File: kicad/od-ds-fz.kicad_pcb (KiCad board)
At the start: 2 copper layers, 42 parts, among them J1 AudioJack2, J2 AudioJack2, U1 TLC274

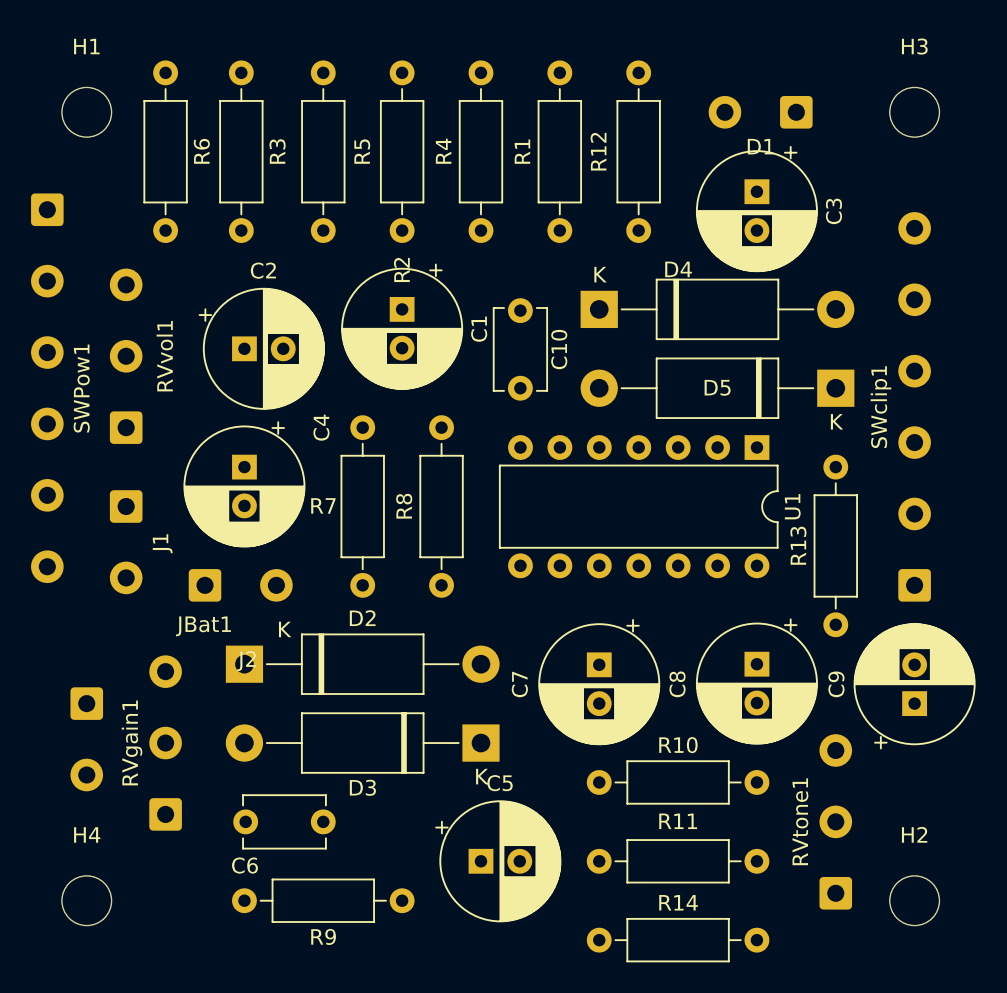
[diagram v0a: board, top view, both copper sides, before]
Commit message: Precise placement
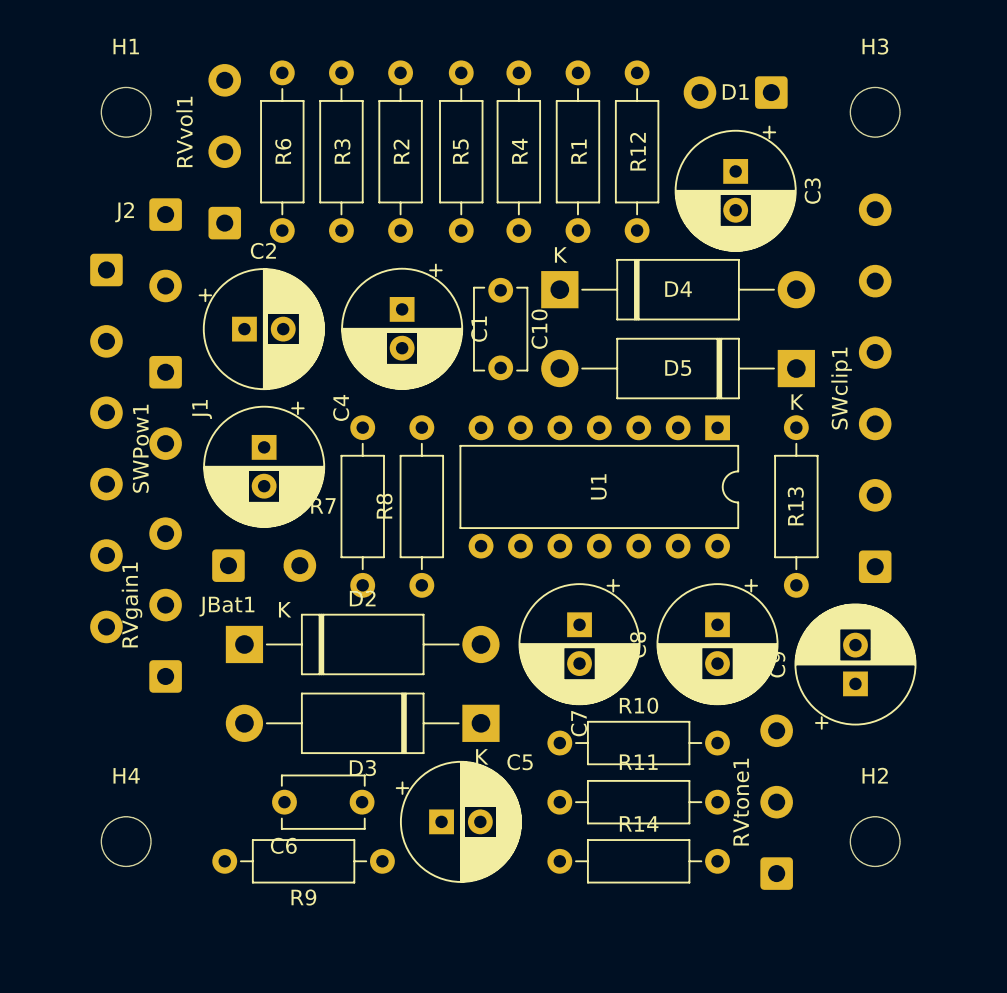
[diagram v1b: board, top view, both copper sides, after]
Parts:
- moved J2 31.9 mm to (127.0, 67.5)
- moved RVvol1 14.6 mm to (130.8, 68.1)
- moved J1 9.02 mm to (127.0, 77.7)
- moved RVgain1 8.89 mm to (127.0, 97.3)
- moved R6 7.52 mm to (134.5, 58.4)
- moved R3 6.45 mm to (138.3, 58.4)
- moved R14 5.68 mm to (152.4, 109.2)
- moved SWPow1 5.44 mm to (123.2, 71.1)
- moved R2 4.98 mm to (142.1, 58.4)
- moved H2 4.58 mm to (172.7, 108.0)
- moved H4 4.58 mm to (124.5, 108.0)
- moved R11 4.58 mm to (162.6, 105.4)
- moved C9 4.02 mm to (171.4, 97.8)
- moved RVtone1 4.02 mm to (166.4, 110.0)
- moved R5 3.81 mm to (146.1, 58.4)
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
